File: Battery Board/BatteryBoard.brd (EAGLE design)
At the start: 40.6 x 80.5 mm, 38 parts, among them IC1 TPS63060DSCT, J0 1725656, J1 1725669, J2 UJ2-MIBH2-4-SMT-TR, J3 MPTC-02-16-02-6.30-XX-X-V, J4 JSTPH2, J5 MPTC-02-04-02-6.30-XX-X-V-LC, Q1 MMBTA56LT1G, Q2 MMBTA56LT1G, U0 STM32L031K4U6, U1 MCP73831T-2ATI_OT, U3 STM809TWX6F

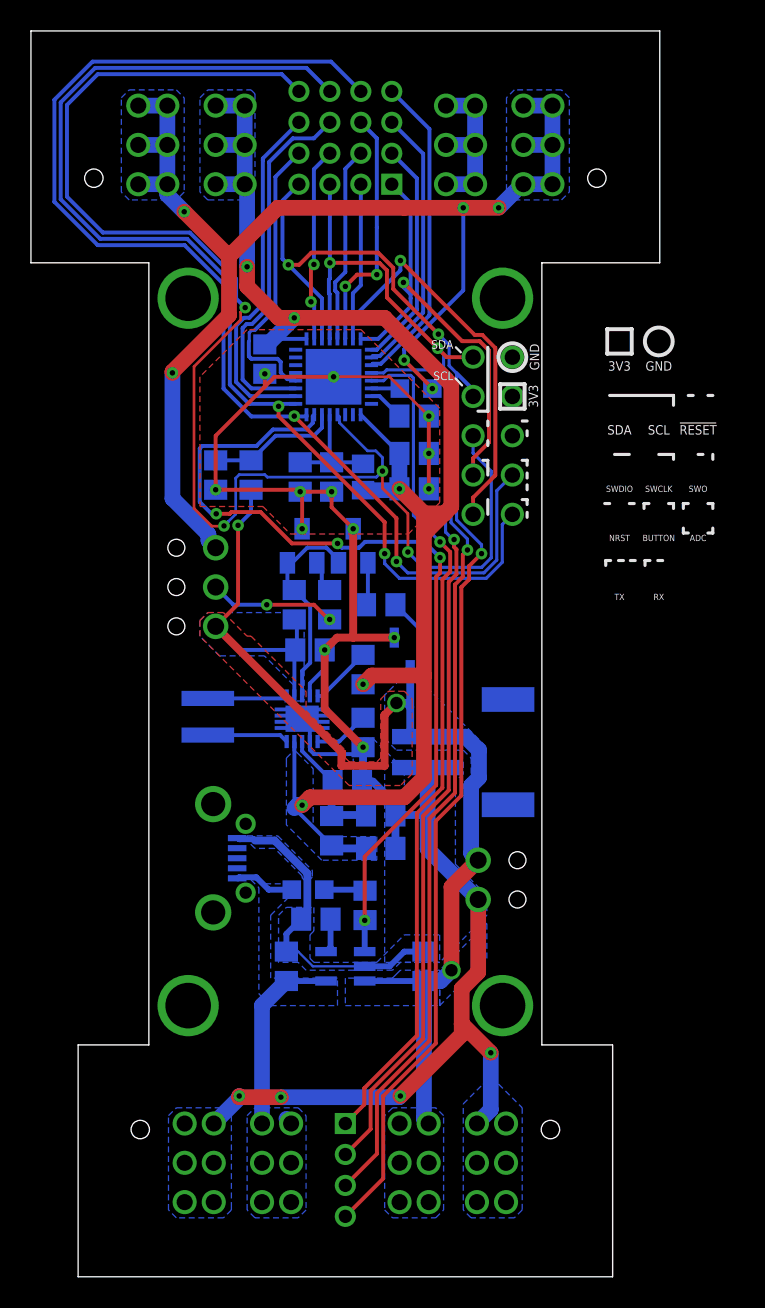
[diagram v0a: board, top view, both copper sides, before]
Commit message: further development. No airwires left
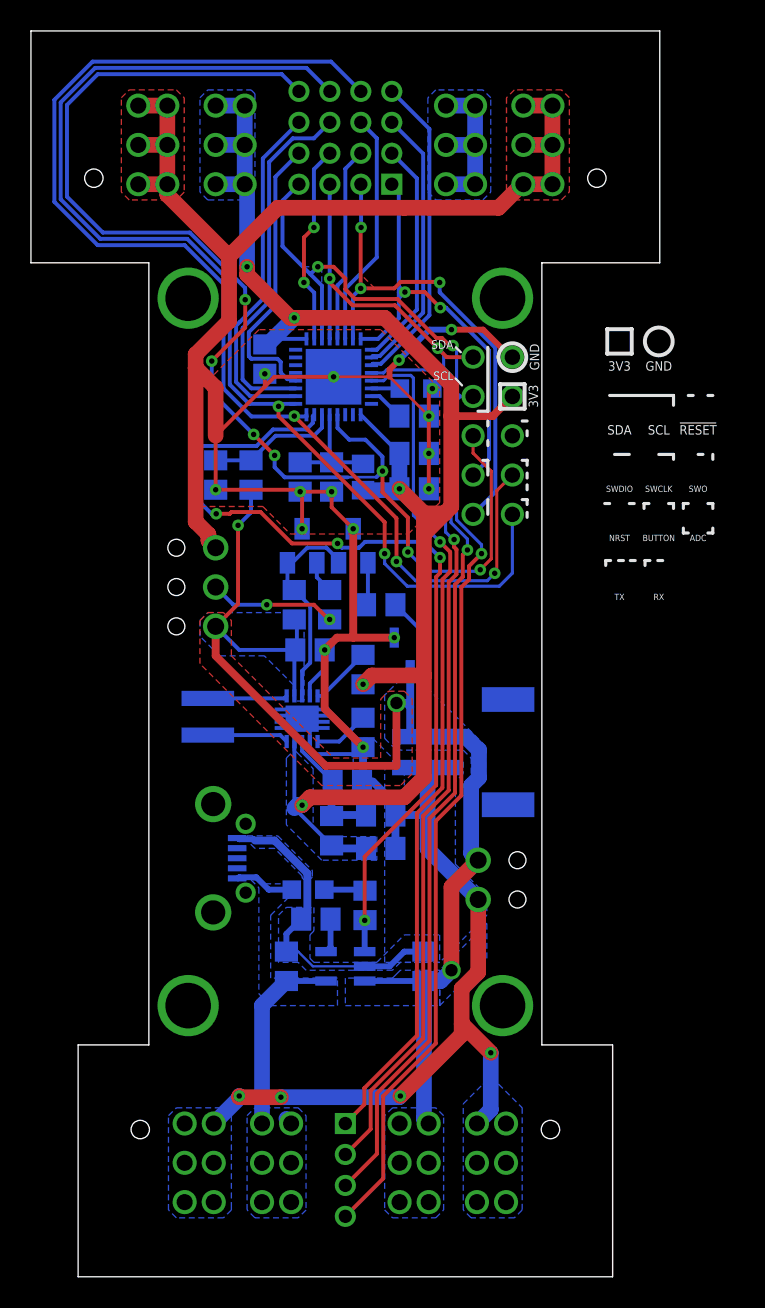
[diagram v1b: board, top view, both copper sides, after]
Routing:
- net NRST: track 92.9 -> 83.8 mm, vias 5 -> 8
- net 3V3: track 102.6 -> 106.6 mm
- net SWDIO: track 35.1 -> 32.6 mm, vias 2 -> 4
- net I2C_SCL: track 88.3 -> 85.9 mm
- net GND: track 229.7 -> 231.5 mm, vias 24 -> 21
- net I2C_SDA: track 81.1 -> 79.7 mm
- net RX: track 74.7 -> 76.0 mm
- net VBAT: track 80.2 -> 81.3 mm
- net TX: track 79.5 -> 80.4 mm, vias 3 -> 4
- net N$4: track 1.83 -> 2.56 mm
- net PA12: track 16.0 -> 15.3 mm, vias 2 -> 0
- net SWCLK: track 29.3 -> 28.8 mm, vias 2 -> 3
- added copper zone on layer 16, net I2C_SCL
- added copper zone on layer 16, net P02
- added copper zone on layer 1, net SWDIO

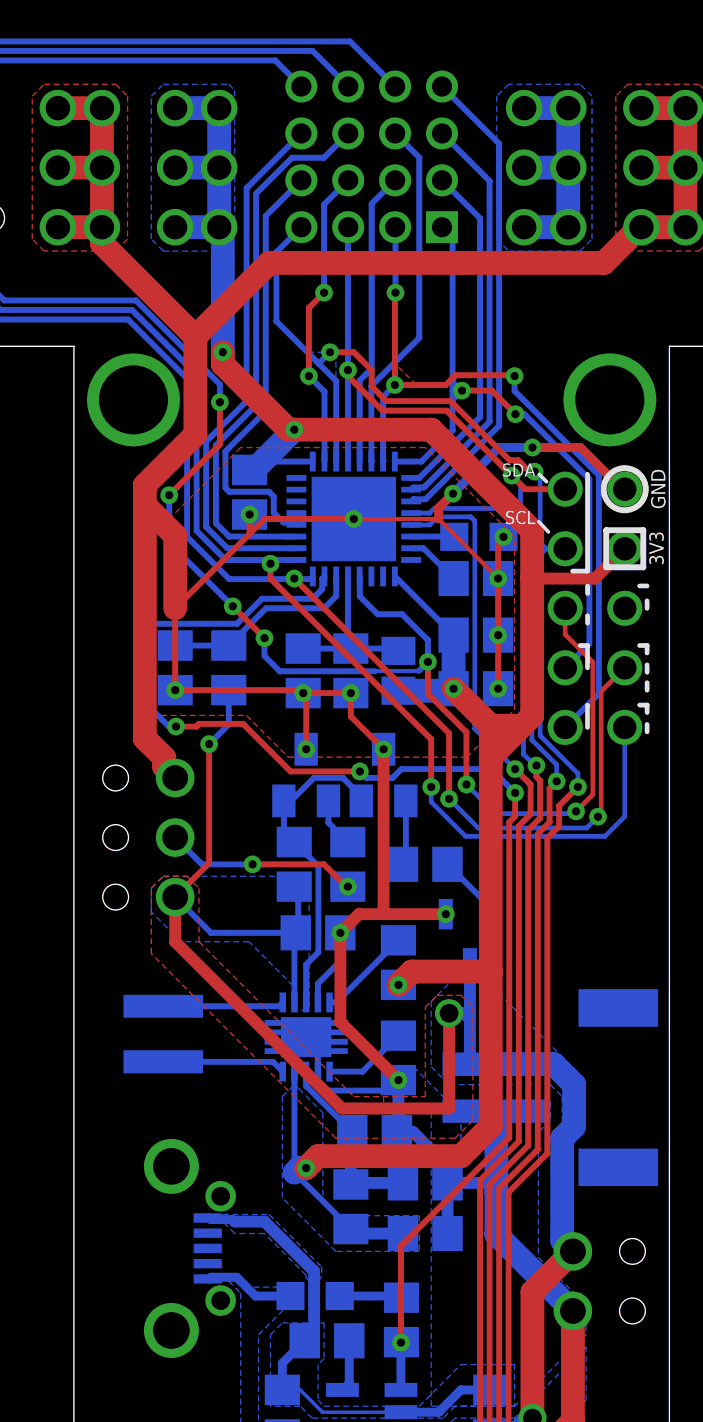
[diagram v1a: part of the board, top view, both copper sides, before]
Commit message: Touch up before final review
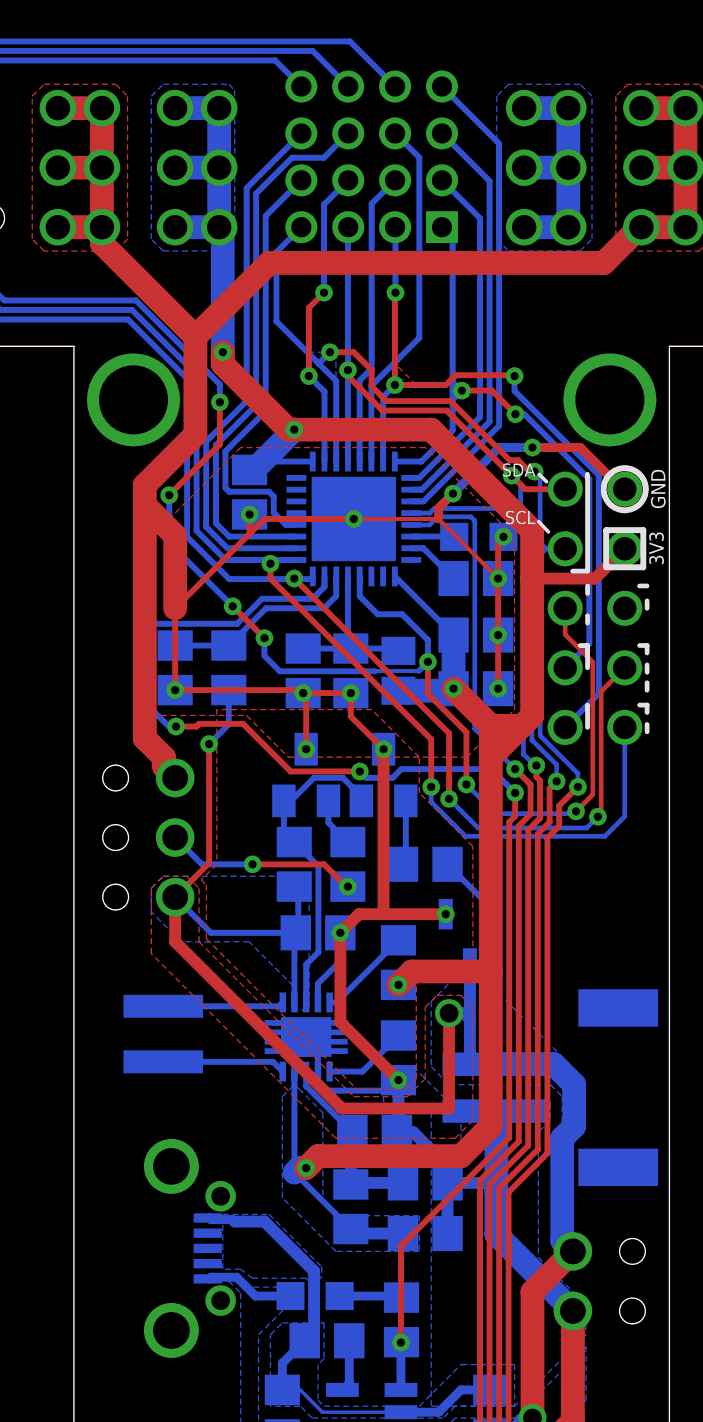
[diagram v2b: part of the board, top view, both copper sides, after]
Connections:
- net GND: now also IC1.11, IC1.12, IC1.13, IC1.14, IC1.15, IC1.16, IC1.17, IC1.18
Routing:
- net GND: track 231.5 -> 243.9 mm
- net 3V3: track 106.6 -> 105.4 mm

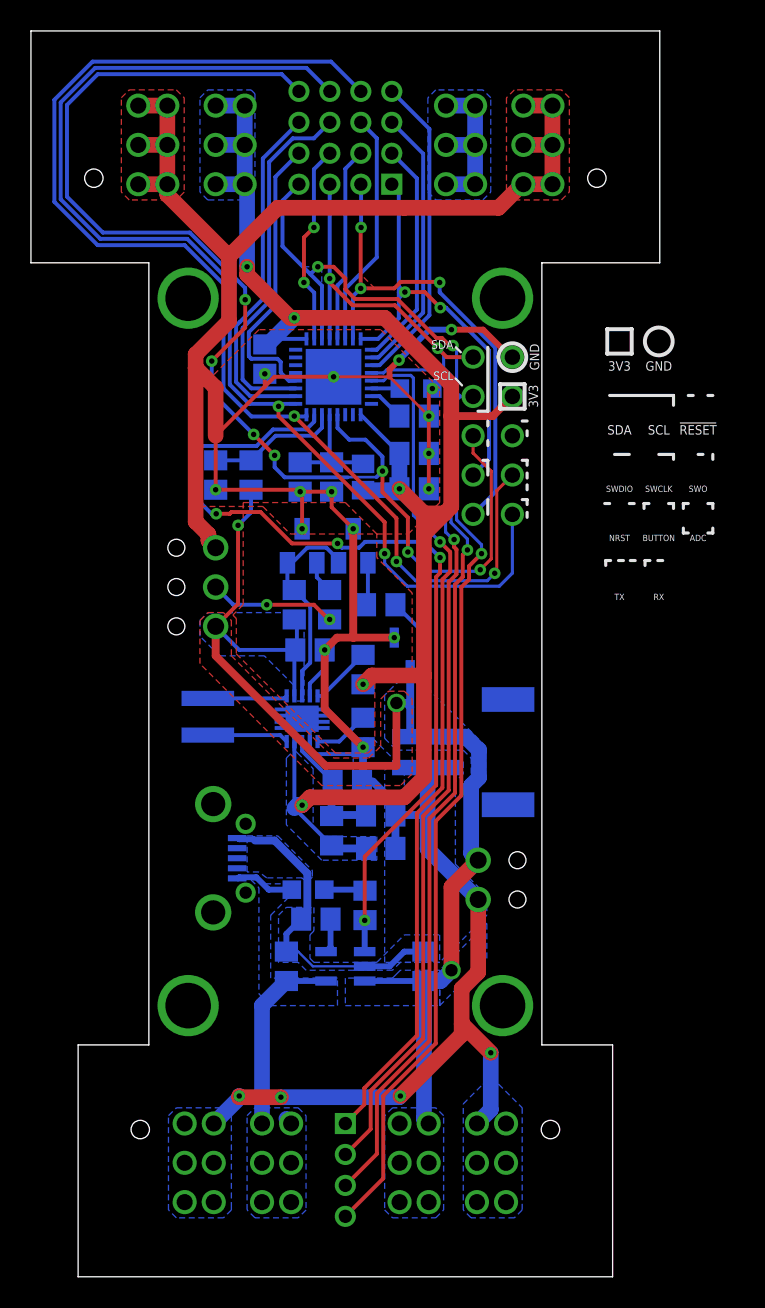
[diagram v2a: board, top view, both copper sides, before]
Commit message: Routed draft
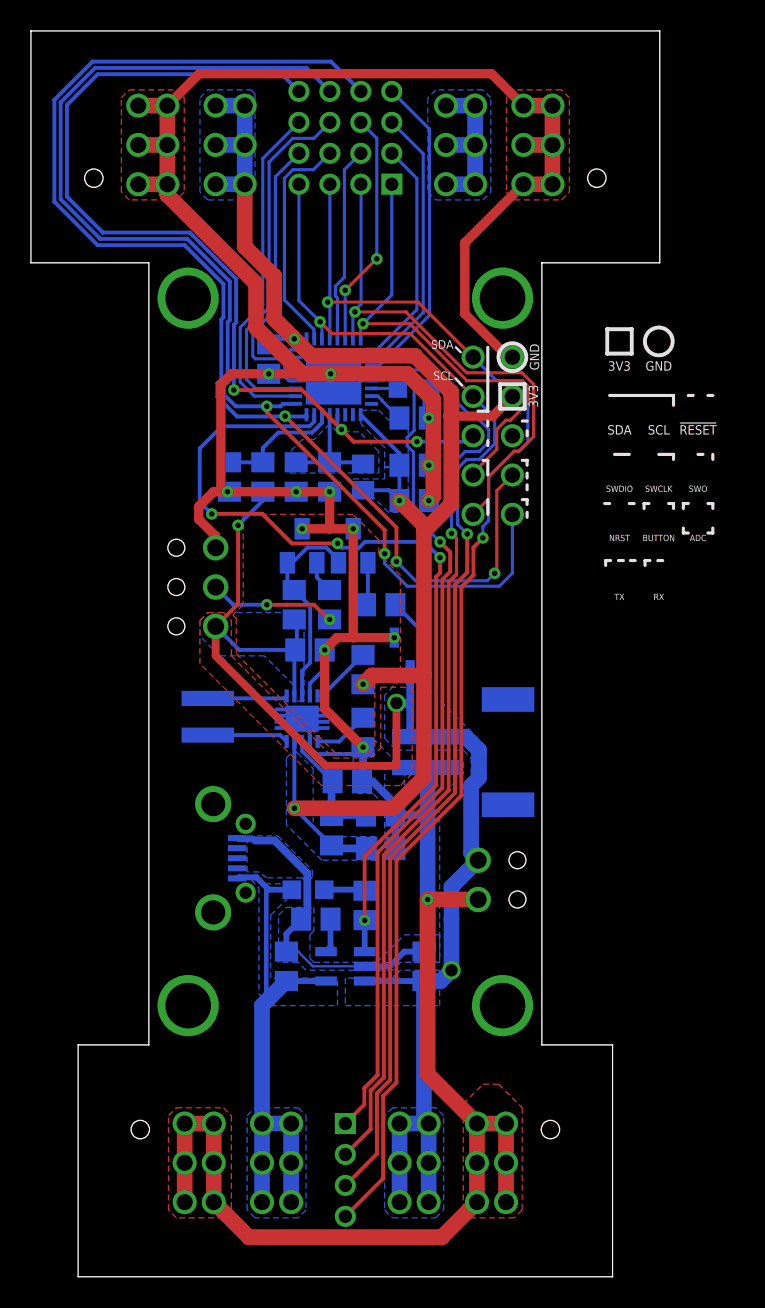
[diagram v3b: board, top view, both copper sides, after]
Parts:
- moved R2 0.90 mm to (-7.49, 11.3)
- moved R1 0.77 mm to (-5.33, 11.3)
- moved C0 0.76 mm to (4.45, 12.1)
- moved C2 0.76 mm to (4.45, 9.78)
- moved C3 0.25 mm to (-3.17, 11.3)
- moved C1 0.25 mm to (-4.95, 18.9)
- moved R0 0.13 mm to (4.45, 15.1)
- moved C4 0.13 mm to (-1.02, 11.3)
- moved LED2 0.13 mm to (4.45, 17.0)
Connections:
- net I2C_SCL: now also J5.C01; no longer J5.D01
- net I2C_SDA: now also J5.D01; no longer J5.C01
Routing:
- net GND: track 243.9 -> 273.5 mm, vias 21 -> 15
- net NRST: track 83.8 -> 61.1 mm, vias 8 -> 4
- net VUSB: track 16.7 -> 35.7 mm
- net VBAT: track 81.3 -> 94.4 mm
- net I2C_SCL: track 85.9 -> 79.1 mm, vias 4 -> 3
- net I2C_SDA: track 79.7 -> 84.2 mm, vias 4 -> 3
- net 3V3: track 105.4 -> 101.8 mm, vias 6 -> 5
- net PB5: track 58.6 -> 61.2 mm
- net PA8: track 13.0 -> 14.8 mm, vias 2 -> 0
- net SWCLK: track 28.8 -> 30.5 mm, vias 3 -> 2
- net SWDIO: track 32.6 -> 34.0 mm, vias 4 -> 2
- net RX: track 76.0 -> 77.2 mm
- net TX: track 80.4 -> 81.5 mm
- net PA12: vias 0 -> 2
- added copper zone on layer 16, net VDDA
- removed copper zone on layer 16, net I2C_SCL
- removed copper zone on layer 1, net SWDIO
